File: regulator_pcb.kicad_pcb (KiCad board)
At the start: 2 copper layers, 28.4 x 9.4 mm, 10 parts, among them J1 Conn_01x02, J2 Conn_01x02, U1 TPS79333-EP

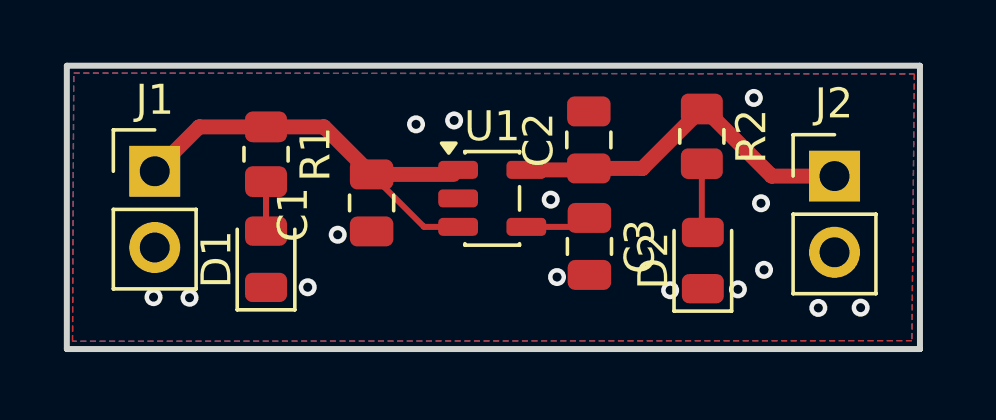
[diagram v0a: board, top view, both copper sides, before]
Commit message: drawing
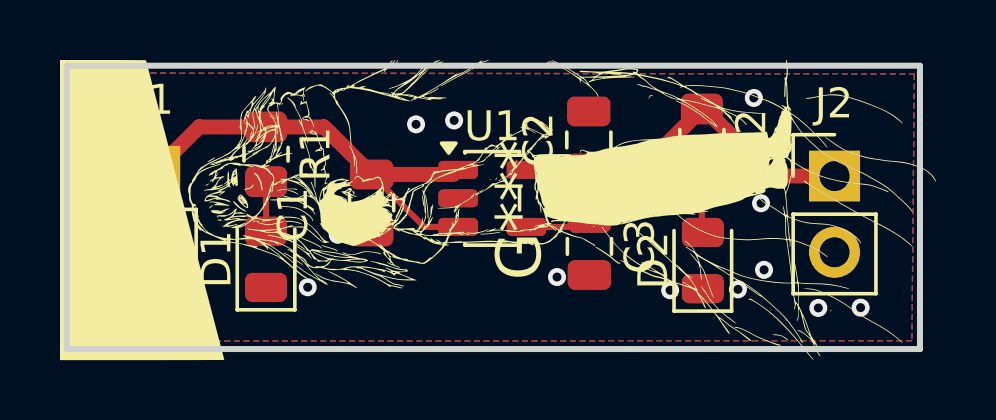
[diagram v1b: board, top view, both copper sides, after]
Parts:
- added G***: LOGO, LOGO, F.Cu at (86.3, 92.1)
